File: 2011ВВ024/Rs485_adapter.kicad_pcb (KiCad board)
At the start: 2 copper layers, 31.5 x 13 mm, 9 parts

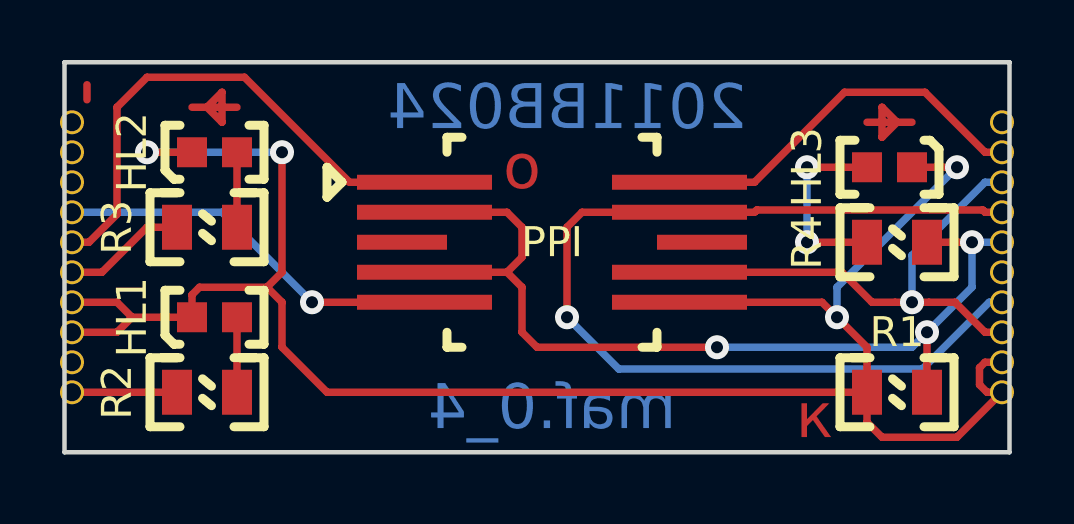
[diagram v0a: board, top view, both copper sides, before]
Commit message: Резонит плакал
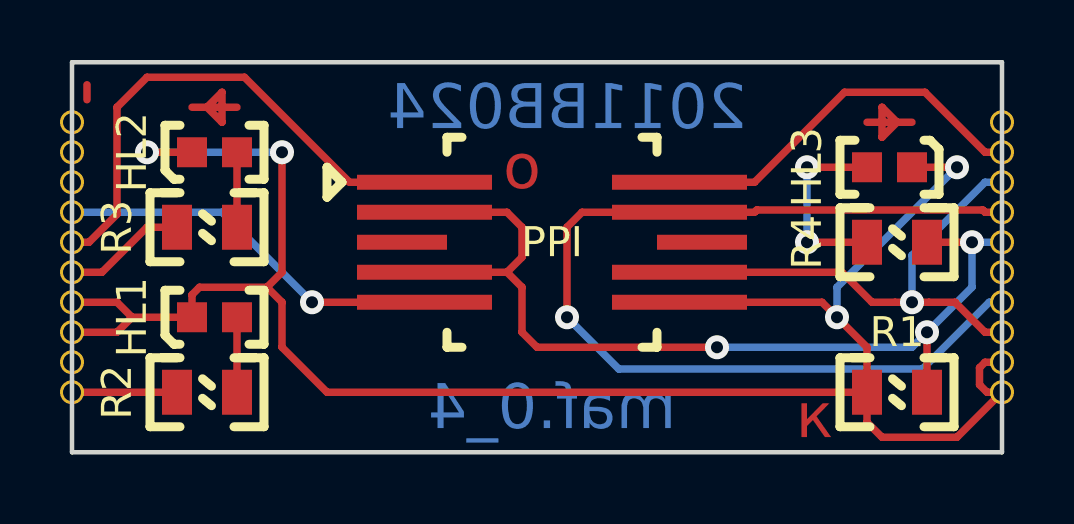
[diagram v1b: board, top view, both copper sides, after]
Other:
- board size 31.5 x 13 mm -> 31 x 13 mm
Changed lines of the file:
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@@
-(kicad_pcb (version 20171130) (host pcbnew "(5.0.0)")
+(kicad_pcb (version 20171130) (host pcbnew "(5.0.2)-1")
   (general
     (thickness 1.6)
@@
       (creategerberjobfile false)
       (excludeedgelayer true)
-      (linewidth 0.200000)
+      (linewidth 0.100000)
       (plotframeref false)
       (viasonmask false)
@@
     (effects (font (size 1.5 1.5) (thickness 0.3)))
   )
-  (gr_line (start 134.25 84.5) (end 134.25 97.5) (layer Edge.Cuts) (width 0.15))
-  (gr_line (start 165.75 97.5) (end 165.75 84.5) (layer Edge.Cuts) (width 0.15))
-  (gr_line (start 165.75 84.5) (end 134.25 84.5) (layer Edge.Cuts) (width 0.15))
-  (gr_line (start 134.25 97.5) (end 165.75 97.5) (layer Edge.Cuts) (width 0.15))
+  (gr_line (start 134.5 84.5) (end 134.5 97.5) (layer Edge.Cuts) (width 0.15))
+  (gr_line (start 165.5 97.5) (end 165.5 84.5) (layer Edge.Cuts) (width 0.15))
+  (gr_line (start 165.5 84.5) (end 134.5 84.5) (layer Edge.Cuts) (width 0.15))
+  (gr_line (start 134.5 97.5) (end 165.5 97.5) (layer Edge.Cuts) (width 0.15))
   (gr_text o (at 149.5 88) (layer F.Cu)
     (effects (font (size 1.5 1.5) (thickness 0.3)))
